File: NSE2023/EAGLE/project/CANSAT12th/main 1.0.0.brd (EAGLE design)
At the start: 77 x 65 mm, 25 parts, among them CN1 DM3AT

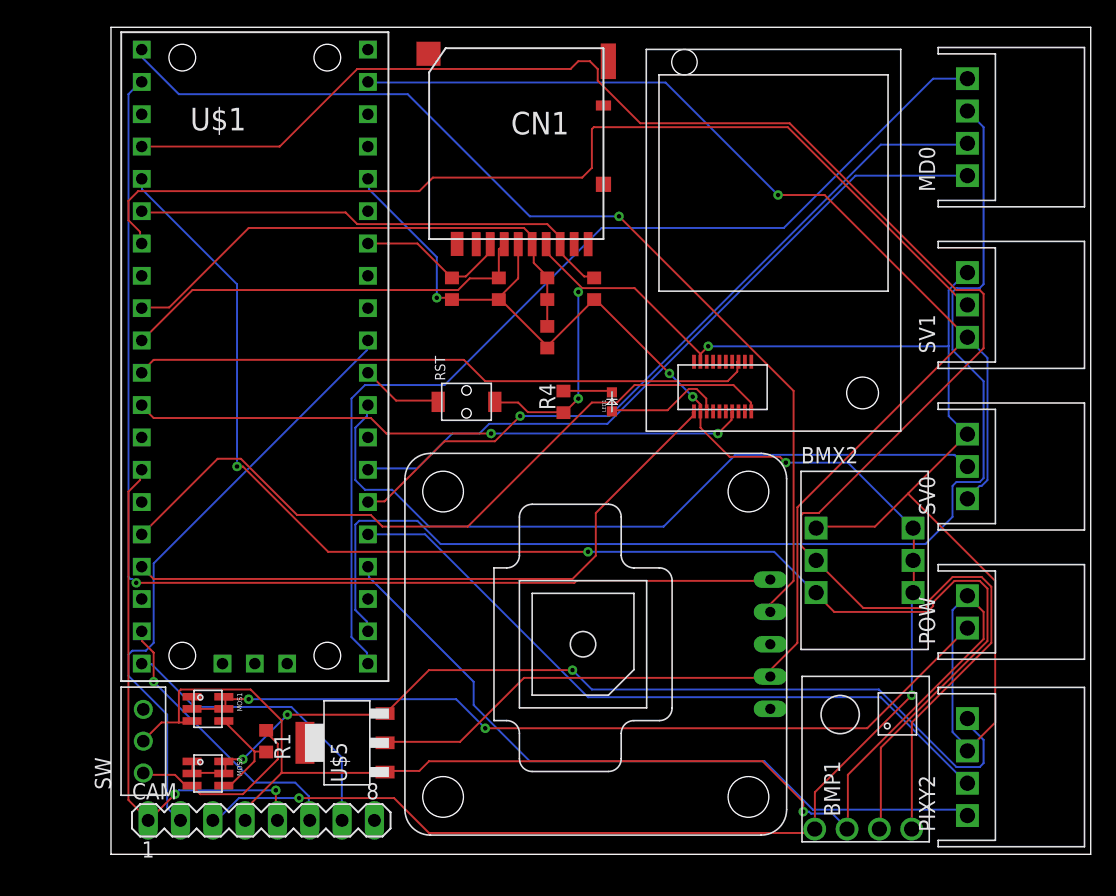
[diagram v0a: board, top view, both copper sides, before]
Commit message: add
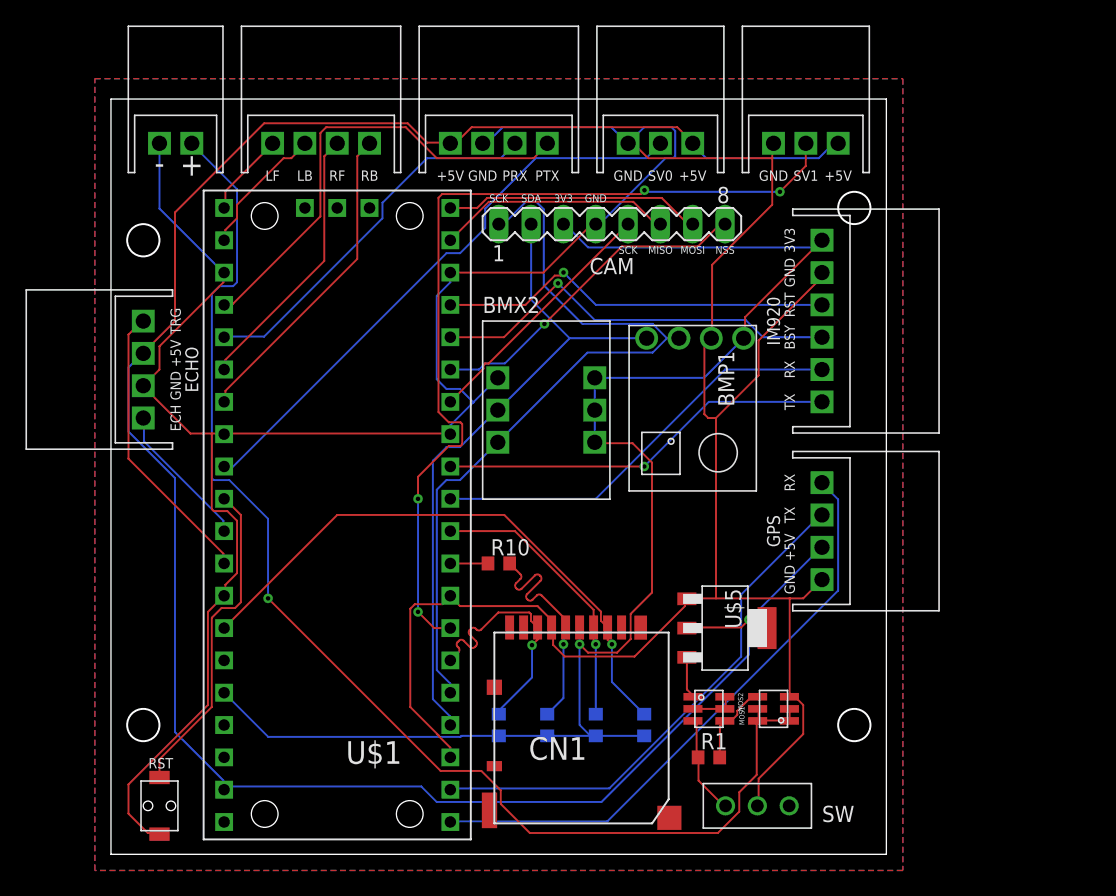
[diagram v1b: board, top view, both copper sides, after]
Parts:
- removed IM: IM920C, IM920:IM920C
- removed LED1: (no value), Chip LED:OSXX1608C1A
- removed R4: 100, rcl:R0603
- removed U$3: AE-GYSFDMAXB, AE-GYSFDMAXB:AE-GYSFDMAXB
- added CON1, CON3: (no value), XR Connector:4PIN_SIDE
- added CON2: (no value), XR Connector:6PIN_SIDE
- moved POW 72.3 mm to (5.08, 55.9), turned to 180 degrees
- moved PIXY2 61.3 mm to (30.5, 55.9), turned to 180 degrees
- moved CAM 54.4 mm to (39.4, 49.5)
- moved MD0 50.8 mm to (16.5, 55.9), turned to 180 degrees
- moved SW 48.5 mm to (50.8, 3.81), turned to 0 degrees
- moved MOS1 44.5 mm to (52.1, 11.4), turned to 90 degrees
- moved CN1 43.2 mm to (36.8, 11.4), turned to 0 degrees
- moved RST 39.9 mm to (3.81, 3.81), turned to 0 degrees
- moved MOS2 39.7 mm to (47.0, 11.4)
- moved R8 37.5 mm to (41.9, 10.2), flipped to the bottom
- moved R7 35.1 mm to (38.1, 10.2), flipped to the bottom
- moved R5 35.1 mm to (30.5, 10.2), flipped to the bottom
- moved SV0 35.0 mm to (43.2, 55.9), turned to 180 degrees
- moved R1 34.8 mm to (47.0, 7.62), turned to 0 degrees
- moved BMP1 31.6 mm to (45.7, 35.6), turned to 270 degrees
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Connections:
- removed net CAM_SCL: U$1.GP27
- removed net CAM_SDA: CAM.2, U$1.GP26
- removed net GND1: U$3.P3
- removed net LED: IM.$P15, LED1.AN
- removed net N$1: CAM.8
- removed net N$3: LED1.CT, R4.2
- new net 1: CN1.CLK, R10.2, R6.2
- new net ECHO: CON3.P$3, U$1.GP26
- new net TRIG: CON3.P$1, U$1.GP27
- net +12V: no longer PIXY2.P$3
- net +3V3: now also CON2.P$6; no longer IM.$P17
- net +5V: now also CON1.P$2, CON3.P$2, PIXY2.P$3; no longer U$3.P4
- net CAM_NSS: now also CAM.8
- net CAM_SCK: no longer CAM.1
- net GND: now also CON1.P$1, CON2.P$5, CON3.P$4, U$1.GND1, U$1.GND2, U$1.GND3, U$1.GND4, U$1.GND6, U$1.GND7, U$1.GND8; no longer IM.$P18, R4.1
- net GPSRX: now also CON1.P$3; no longer U$3.P2
- net GPSTX: now also CON1.P$4; no longer U$3.P1
- net IM_BUSY: now also CON2.P$3; no longer IM.$P1
- net IM_RESET: now also CON2.P$4; no longer IM.$P19
- net IM_RX: now also CON2.P$2; no longer IM.$P6
- net IM_TX: now also CON2.P$1; no longer IM.$P7
- net SCK: no longer CN1.CLK, R10.2, R6.2
- net SCL: now also CAM.1
- net SDA: now also CAM.2
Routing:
- net SDA: track 143.6 -> 52.4 mm
- net LB: track 95.1 -> 10.6 mm
- net LF: track 80.2 -> 6.65 mm
- net GND: track 214.7 -> 282.8 mm, vias 4 -> 0
- net +12V: track 74.6 -> 7.91 mm, vias 3 -> 0
- net SCL: track 113.3 -> 62.2 mm, vias 2 -> 0
- net GPSTX: track 90.2 -> 41.1 mm, vias 1 -> 0
- net CAM_SDA: track 47.9 -> 0.00 mm
- net SCK: track 41.2 -> 2.96 mm
- net RF: track 58.8 -> 21.5 mm, vias 1 -> 0
- net +5V: track 135.1 -> 170.7 mm
- net GPSRX: track 80.8 -> 47.0 mm, vias 1 -> 0
- net NSS: track 12.2 -> 45.9 mm, vias 0 -> 1
- net N$8: track 67.4 -> 99.4 mm, vias 2 -> 1
- net RB: track 56.7 -> 25.0 mm
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- added copper zone on layer 1, net GND
- added copper zone on layer 16, net GND
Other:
- board size 77 x 65 mm -> 60.9 x 59.4 mm
- board text added: "+"
- board text added: "+5V"
- board text added: "-"
- board text added: "3V3"
- board text added: "BSY"
- board text added: "CAM"
- board text added: "ECH"
- board text added: "ECHO"
- board text added: "GND"
- board text added: "GPS"
- board text added: "IM920"
- board text added: "LB"
- board text added: "LF"
- board text added: "MISO"
- board text added: "MOSI"
- board text added: "NSS"
- board text added: "PRX"
- board text added: "PTX"
- board text added: "RB"
- board text added: "RF"
- board text added: "RST"
- board text added: "RX"
- board text added: "SCK"
- board text added: "SDA"
- board text added: "SV0"
- board text added: "SV1"
- board text added: "TRG"
- board text added: "TX"
